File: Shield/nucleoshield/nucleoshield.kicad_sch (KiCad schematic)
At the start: 21 parts, among them J1 Conn_02x19_Odd_Even, J2 Conn_02x19_Odd_Even

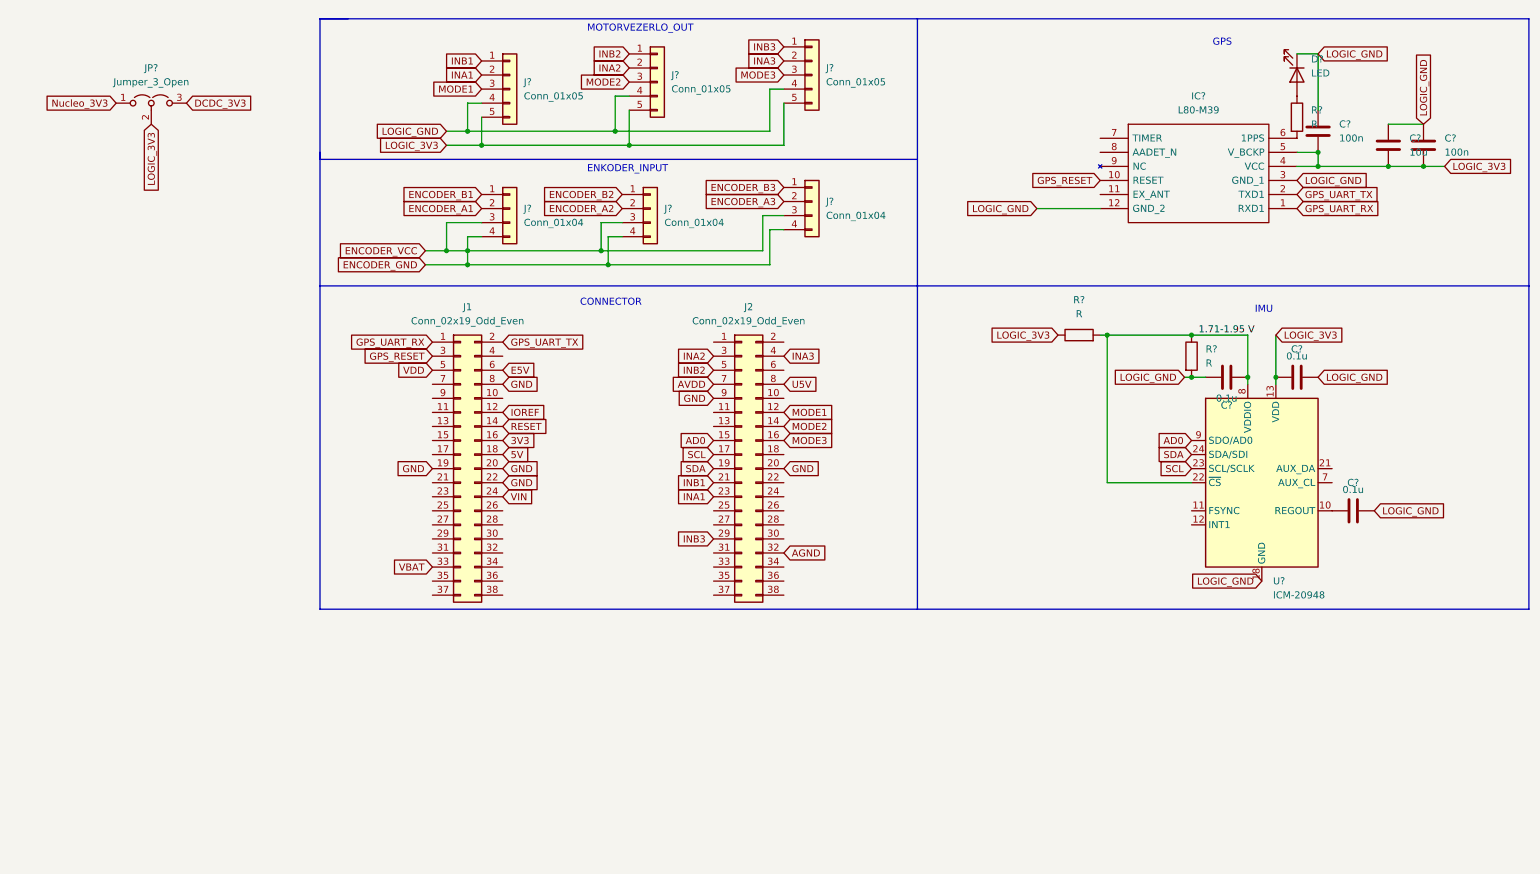
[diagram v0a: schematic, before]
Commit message: Nucleo shield
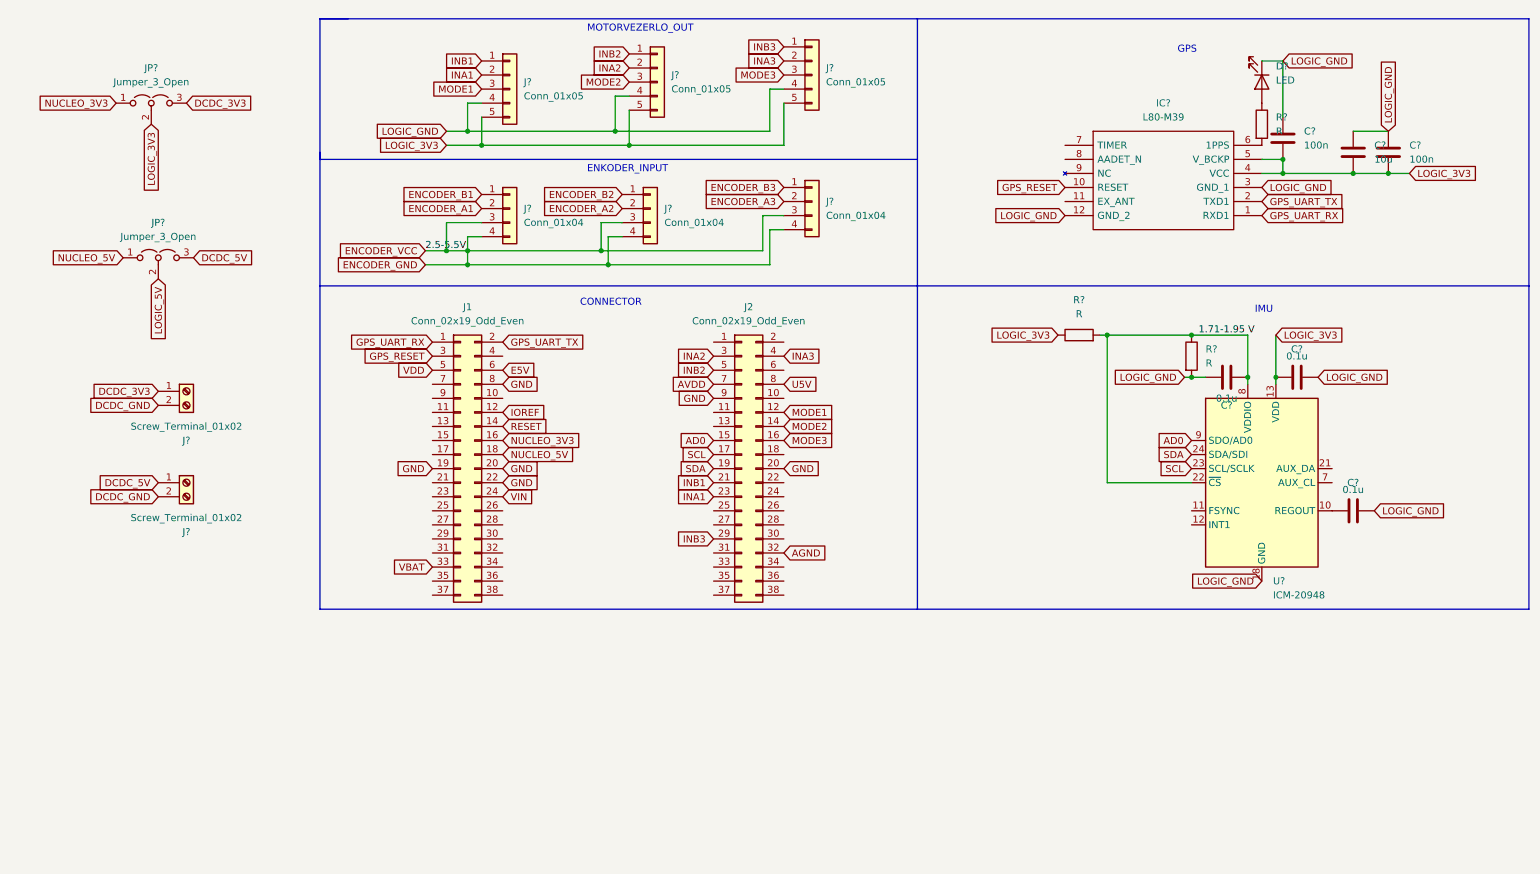
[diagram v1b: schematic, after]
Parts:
- added J? (x2): Screw_Terminal_01x02, Connector_TE-Connectivity:TE_826576-2_1x02_P3.96mm_Vertical, symbol Connector:Screw_Terminal_01x02
- added JP?: Jumper_3_Open, symbol Jumper:Jumper_3_Open
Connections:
- net Nucleo_3V3 is gone; now on net NUCLEO_3V3: JP?.1 (A)
- net DCDC_3V3: now also J?.1 (Pin_1)
- net 3V3 renamed NUCLEO_3V3
- net 5V renamed NUCLEO_5V
- net NUCLEO_5V: now also JP?.1 (A)
- new net DCDC_5V: J?.1 (Pin_1), JP?.3 (B)
- new net DCDC_GND: J?.2 (Pin_2), J?.2 (Pin_2)
- new net LOGIC_5V: JP?.2 (C)
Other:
- moved on the sheet: C?, D?, IC?, R?

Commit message: Schematic and pcb ready
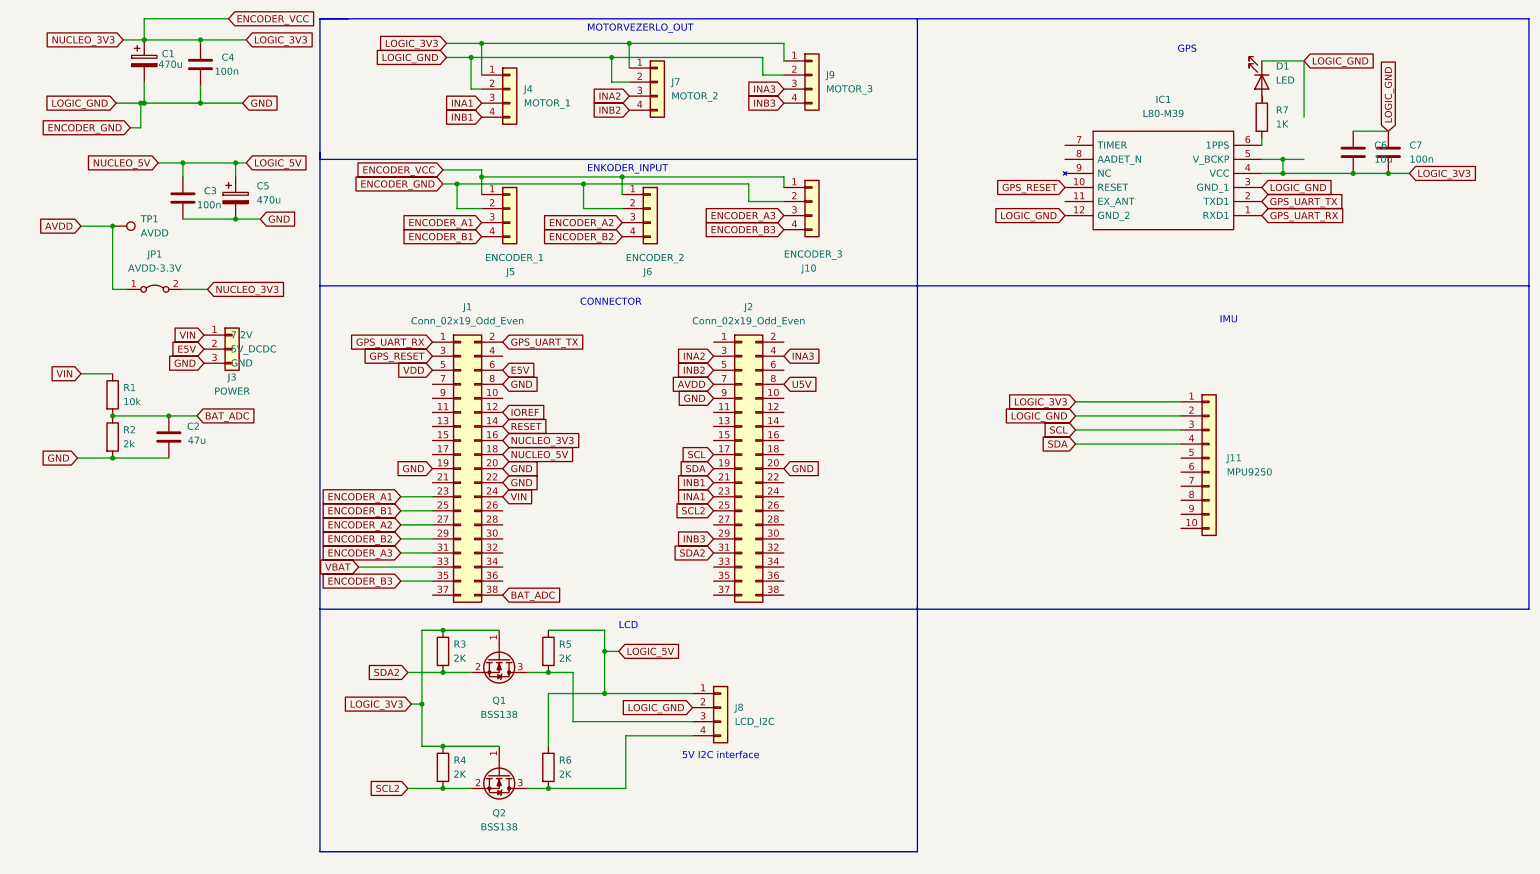
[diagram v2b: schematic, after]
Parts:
- removed C?: 100n, symbol Device:C
- removed C? (x3): 0.1u, symbol Device:C
- removed IC?: L80-M39, L80-M39, symbol L80-M39:L80-M39
- removed J? (x3): Conn_01x05, Connector_PinSocket_2.54mm:PinSocket_1x05_P2.54mm_Vertical, symbol Connector_Generic:Conn_01x05
- removed J? (x2): Screw_Terminal_01x02, Connector_TE-Connectivity:TE_826576-2_1x02_P3.96mm_Vertical, symbol Connector:Screw_Terminal_01x02
- removed JP? (x2): Jumper_3_Open, symbol Jumper:Jumper_3_Open
- removed R? (x2): R, symbol Device:R
- removed U?: ICM-20948, Sensor_Motion:InvenSense_QFN-24_3x3mm_P0.4mm, symbol Sensor_Motion:ICM-20948
- added C1, C5: 470u, Capacitor_THT:CP_Radial_D8.0mm_P3.50mm, symbol Device:C_Polarized
- added C2: 47u, Capacitor_SMD:C_1206_3216Metric, symbol Device:C
- added C3, C4: 100n, Capacitor_SMD:C_1206_3216Metric, symbol Device:C
- added IC1: L80-M39, componentLib:L80-M39, symbol L80-M39:L80-M39
- added J11: MPU9250, Connector_PinHeader_2.54mm:PinHeader_1x10_P2.54mm_Vertical, symbol Connector_Generic:Conn_01x10
- added J3: POWER, Connector_PinHeader_2.54mm:PinHeader_1x03_P2.54mm_Vertical, symbol Connector_Generic:Conn_01x03
- added J4: MOTOR_1, Connector_PinSocket_2.54mm:PinSocket_1x04_P2.54mm_Vertical, symbol Connector_Generic:Conn_01x04
- added J7: MOTOR_2, Connector_PinSocket_2.54mm:PinSocket_1x04_P2.54mm_Vertical, symbol Connector_Generic:Conn_01x04
- added J8: LCD_I2C, Connector_PinSocket_2.54mm:PinSocket_1x04_P2.54mm_Vertical, symbol Connector_Generic:Conn_01x04
- added J9: MOTOR_3, Connector_PinSocket_2.54mm:PinSocket_1x04_P2.54mm_Vertical, symbol Connector_Generic:Conn_01x04
- added JP1: AVDD-3.3V, Jumper:SolderJumper-2_P1.3mm_Bridged2Bar_Pad1.0x1.5mm, symbol Jumper:Jumper_2_Bridged
- added Q1, Q2: BSS138, Package_TO_SOT_SMD:SOT-23, symbol Transistor_FET:BSS138
- added R1: 10k, Resistor_SMD:R_0805_2012Metric, symbol Device:R
- added R2: 2k, Resistor_SMD:R_0805_2012Metric, symbol Device:R
- added R3, R4, R5, R6: 2K, Resistor_SMD:R_0805_2012Metric, symbol Device:R
- added TP1: AVDD, TestPoint:TestPoint_THTPad_1.0x1.0mm_Drill0.5mm, symbol Connector:TestPoint
- C6, C7: renamed from C?; footprint (none) -> Capacitor_SMD:C_1206_3216Metric
- D1: renamed from D?; footprint (none) -> LED_SMD:LED_0805_2012Metric
- J10: renamed from J?; value Conn_01x04 -> ENCODER_3; footprint (none) -> Connector_PinSocket_2.54mm:PinSocket_1x04_P2.54mm_Vertical
- J5: renamed from J?; value Conn_01x04 -> ENCODER_1
- J6: renamed from J?; value Conn_01x04 -> ENCODER_2; footprint (none) -> Connector_PinSocket_2.54mm:PinSocket_1x04_P2.54mm_Vertical
- R7: renamed from R?; value R -> 1K; footprint (none) -> Resistor_SMD:R_0805_2012Metric
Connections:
- net GND is gone; now on net ENCODER_GND: J1.19 (Pin_19), J1.20 (Pin_20), J1.22 (Pin_22), J1.8 (Pin_8), J2.20 (Pin_20), J2.9 (Pin_9)
- net LOGIC_GND is gone; now on net ENCODER_GND: C6.1, C7.1, D1.1 (K)
- net NUCLEO_3V3 is gone; now on net ENCODER_VCC: J1.16 (Pin_16)
- net NUCLEO_5V is gone; now on net LOGIC_5V: J1.18 (Pin_18)
- net AVDD: now also JP1.1 (A), TP1.1
- net E5V: now also J3.2 (5V_DCDC)
- net ENCODER_A1: now also J1.23 (Pin_23), J5.3 (Pin_3); no longer J5.2 (Pin_2)
- net ENCODER_A2: now also J1.27 (Pin_27), J6.3 (Pin_3); no longer J6.2 (Pin_2)
- net ENCODER_A3: now also J1.31 (Pin_31), J10.3 (Pin_3); no longer J10.2 (Pin_2)
- net ENCODER_B1: now also J1.25 (Pin_25), J5.4 (Pin_4); no longer J5.1 (Pin_1)
- net ENCODER_B2: now also J1.29 (Pin_29), J6.4 (Pin_4); no longer J6.1 (Pin_1)
- net ENCODER_B3: now also J1.35 (Pin_35), J10.4 (Pin_4); no longer J10.1 (Pin_1)
- net ENCODER_GND: now also J10.2 (Pin_2), J5.2 (Pin_2), J6.2 (Pin_2), C1.2, C2.1, C3.2, C4.2, C5.2, IC1.12 (GND_2), IC1.3 (GND_1), J11.2 (Pin_2), J3.3 (GND), J4.2 (Pin_2), J7.2 (Pin_2), J8.2 (Pin_2), J9.2 (Pin_2), R2.2; no longer J10.3 (Pin_3), J10.4 (Pin_4), J5.3 (Pin_3), J5.4 (Pin_4), J6.3 (Pin_3), J6.4 (Pin_4)
- net GPS_RESET: now also IC1.10 (RESET)
- net GPS_UART_RX: now also IC1.1 (RXD1)
- net GPS_UART_TX: now also IC1.2 (TXD1)
- net INA1: now also J4.3 (Pin_3)
- net INA2: now also J7.3 (Pin_3)
- net INA3: now also J9.3 (Pin_3)
- net INB1: now also J4.4 (Pin_4)
- net INB2: now also J7.4 (Pin_4)
- net INB3: now also J9.4 (Pin_4)
- net LOGIC_5V: now also C3.1, C5.1, J8.1 (Pin_1), R5.1, R6.1
- net SCL: now also J11.3 (Pin_3)
- net SDA: now also J11.4 (Pin_4)
- net VIN: now also J3.1 (7.2V), R1.1
- net at R7.2: now also IC1.6 (1PPS)
- net BAT_ADC: now reaches J1.38 (Pin_38)
- net BAT_ADC: now also C2.2, R1.2, R2.1
- net SCL2: now reaches J2.25 (Pin_25)
- net SCL2: now also Q2.2 (S), R4.2
- net SDA2: now reaches J2.31 (Pin_31)
- net SDA2: now also Q1.2 (S), R3.2
- net AD0: no longer names the net of J2.15 (Pin_15)
- net AGND: no longer names the net of J2.32 (Pin_32)
- net LOGIC_3V3 renamed ENCODER_VCC
- net ENCODER_VCC: now also J10.1 (Pin_1), J5.1 (Pin_1), J6.1 (Pin_1), C1.1, C4.1, IC1.4 (VCC), IC1.5 (V_BCKP), J11.1 (Pin_1), J4.1 (Pin_1), J7.1 (Pin_1), J9.1 (Pin_1), JP1.2 (B), Q1.1 (G), Q2.1 (G), R3.1, R4.1
- net MODE1: no longer names the net of J2.12 (Pin_12)
- net MODE2: no longer names the net of J2.14 (Pin_14)
- net MODE3: no longer names the net of J2.16 (Pin_16)
- new net: J8.3 (Pin_3), Q1.3 (D), R5.2
- new net: J8.4 (Pin_4), Q2.3 (D), R6.2
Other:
- note added: "5V I2C interface"
- note added: "LCD"
- moved on the sheet: R7

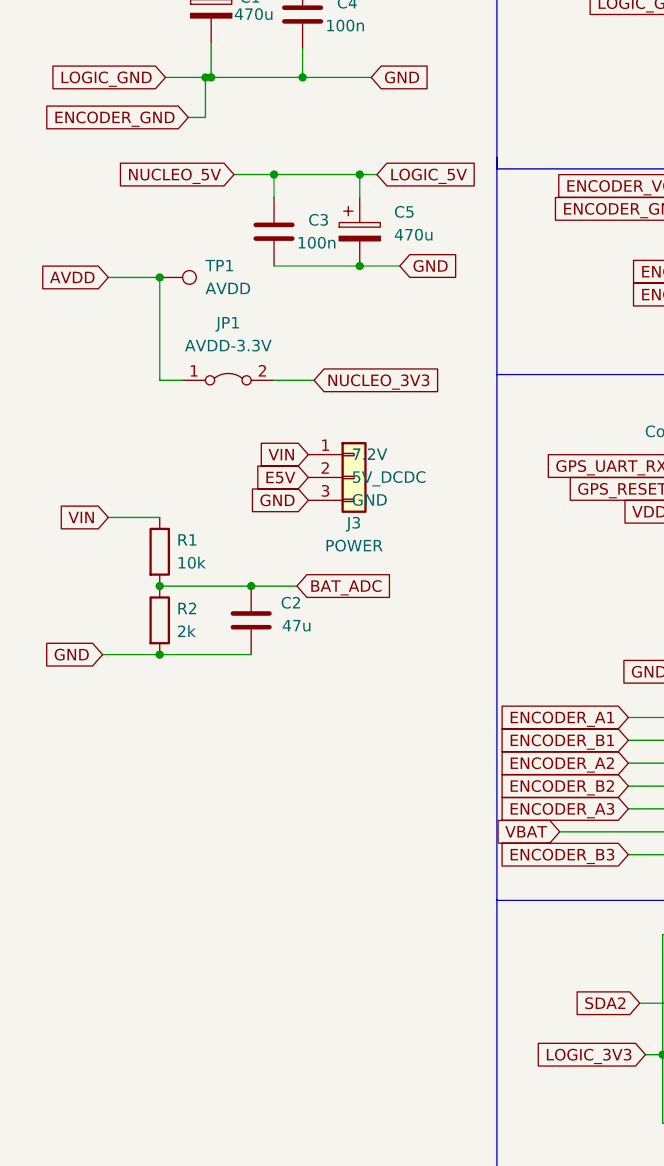
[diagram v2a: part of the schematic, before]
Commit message: power modifications
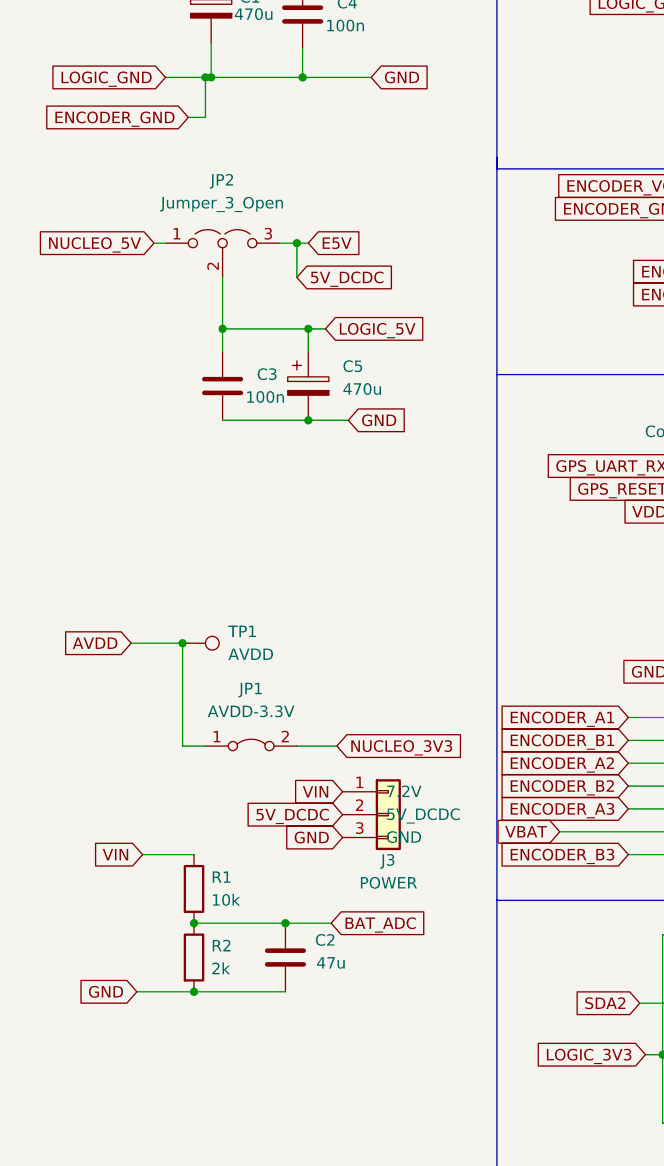
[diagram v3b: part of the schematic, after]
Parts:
- added JP2: Jumper_3_Open, Connector_PinSocket_2.54mm:PinSocket_1x03_P2.54mm_Vertical, symbol Jumper:Jumper_3_Open
- J10, J4, J5, J6, J7, J8, J9: footprint Connector_PinSocket_2.54mm:PinSocket_1x04_P2.54mm_Vertical -> Connector_JST:JST_EH_B4B-EH-A_1x04_P2.50mm_Vertical
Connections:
- net LOGIC_5V: now also JP2.2 (C); no longer J1.18 (Pin_18)
- net E5V renamed 5V_DCDC
- net 5V_DCDC: now also JP2.3 (B)
- new net NUCLEO_5V: J1.18 (Pin_18), JP2.1 (A)
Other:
- moved on the sheet: C2, C3, C5, J3, JP1, R1, R2, TP1

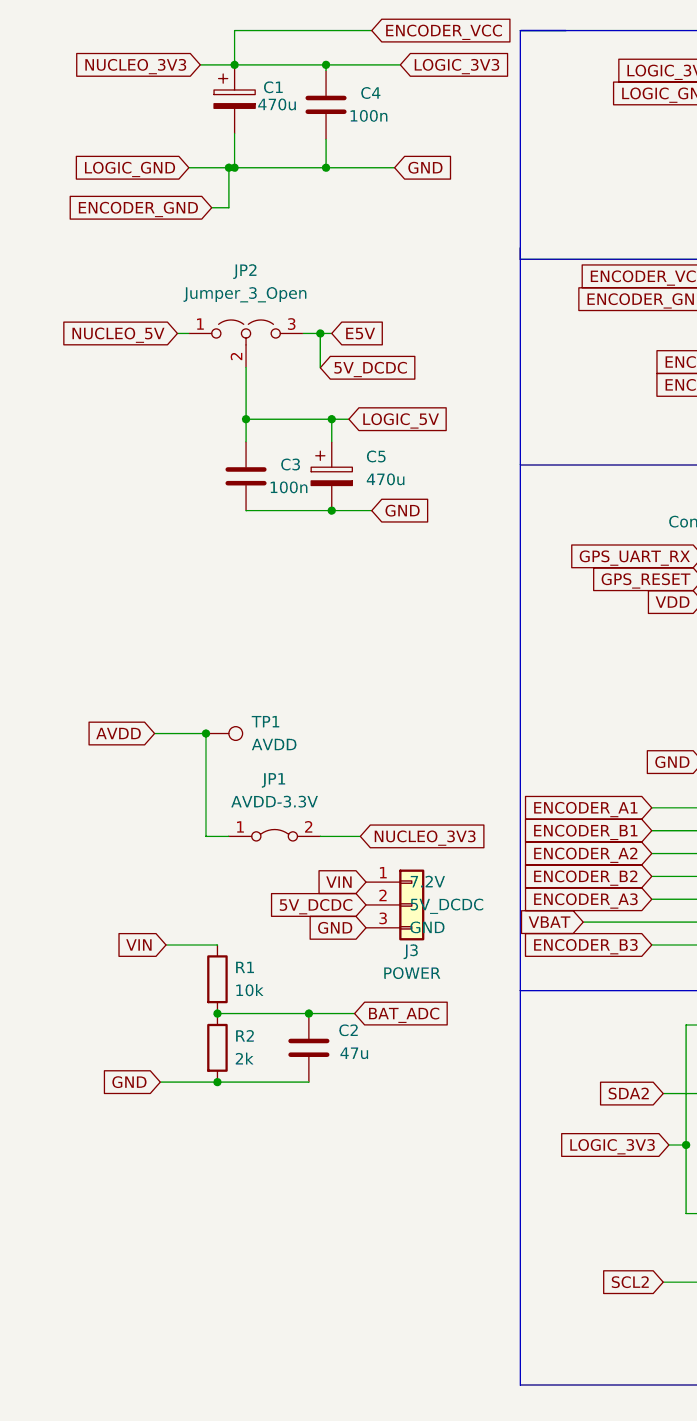
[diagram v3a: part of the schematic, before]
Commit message: Power connector
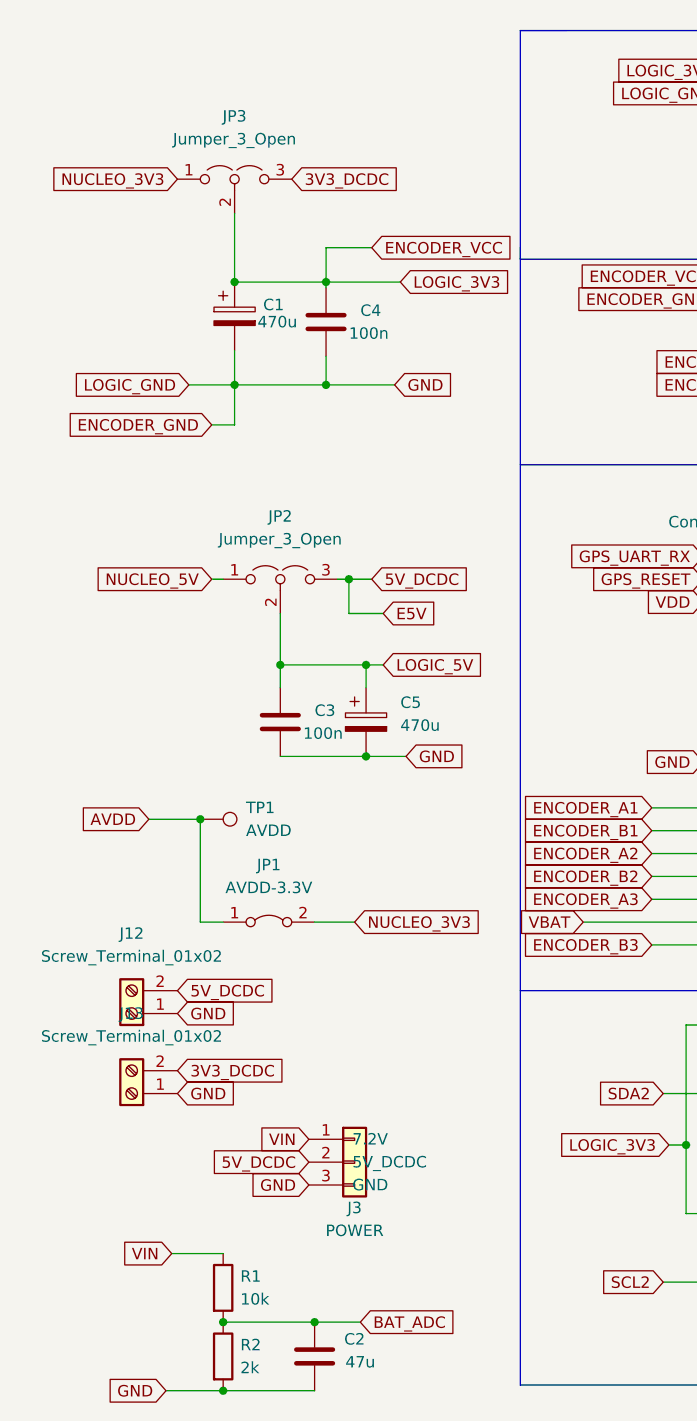
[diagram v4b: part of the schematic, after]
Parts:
- added J12, J13: Screw_Terminal_01x02, TerminalBlock:TerminalBlock_Altech_AK300-2_P5.00mm, symbol Connector:Screw_Terminal_01x02
- added JP3: Jumper_3_Open, Connector_PinSocket_2.54mm:PinSocket_1x03_P2.54mm_Vertical, symbol Jumper:Jumper_3_Open
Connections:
- net 5V_DCDC: now also J12.2 (Pin_2)
- net ENCODER_GND: now also J12.1 (Pin_1), J13.1 (Pin_1)
- net ENCODER_VCC: now also JP3.2 (C); no longer J1.16 (Pin_16), JP1.2 (B)
- new net 3V3_DCDC: J13.2 (Pin_2), JP3.3 (B)
- new net NUCLEO_3V3: J1.16 (Pin_16), JP1.2 (B), JP3.1 (A)
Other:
- moved on the sheet: C1, C2, C3, C4, C5, J3, JP1, JP2, R1, R2, TP1
